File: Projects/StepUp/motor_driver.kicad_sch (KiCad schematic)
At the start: 39 parts, among them J4 AST250404, Q1 BSS84, Q2 2N7002-7-F, U4 TMC2300-LA

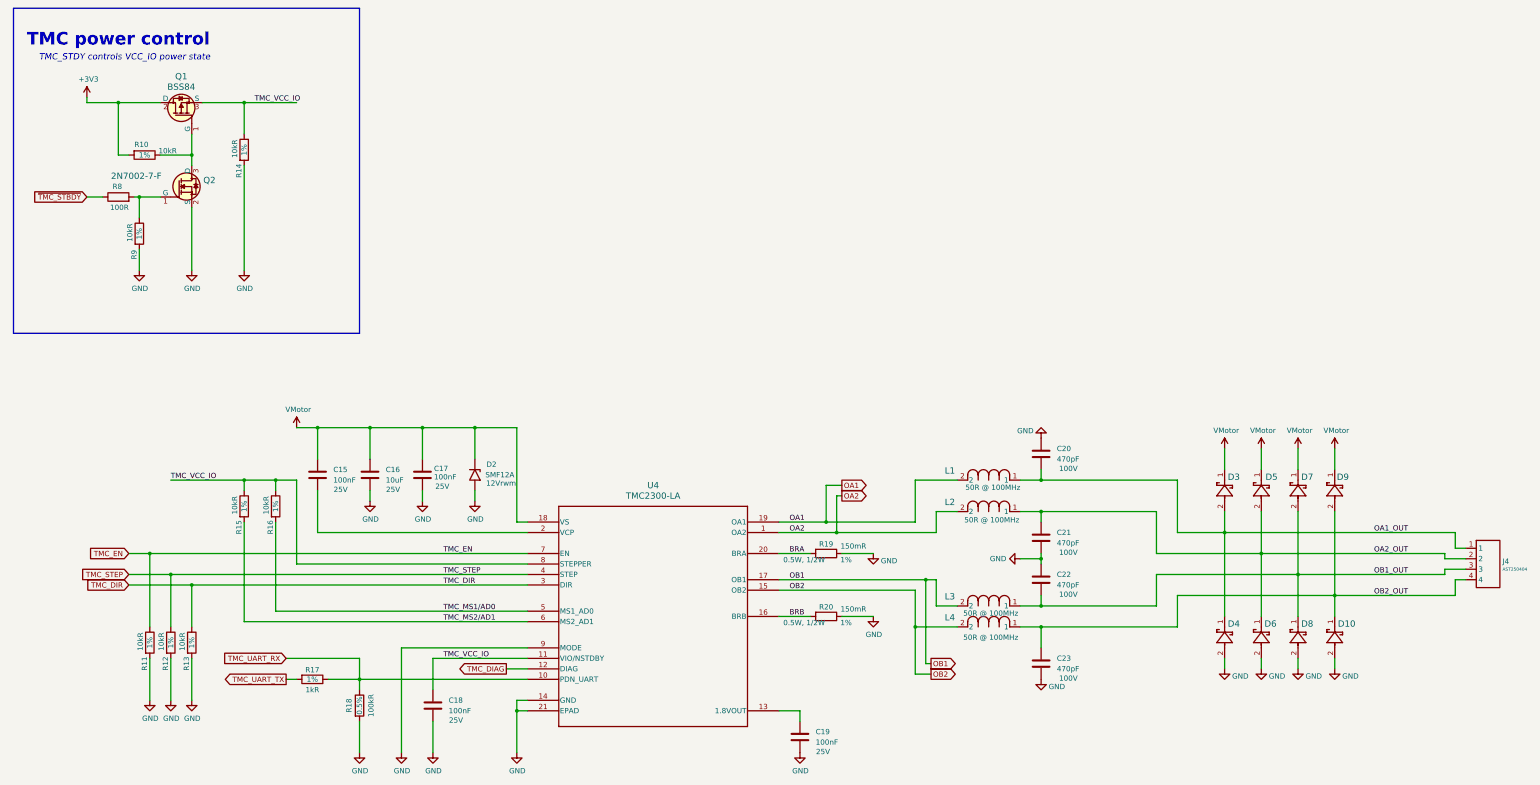
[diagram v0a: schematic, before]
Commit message: feat(layout): Layout begins
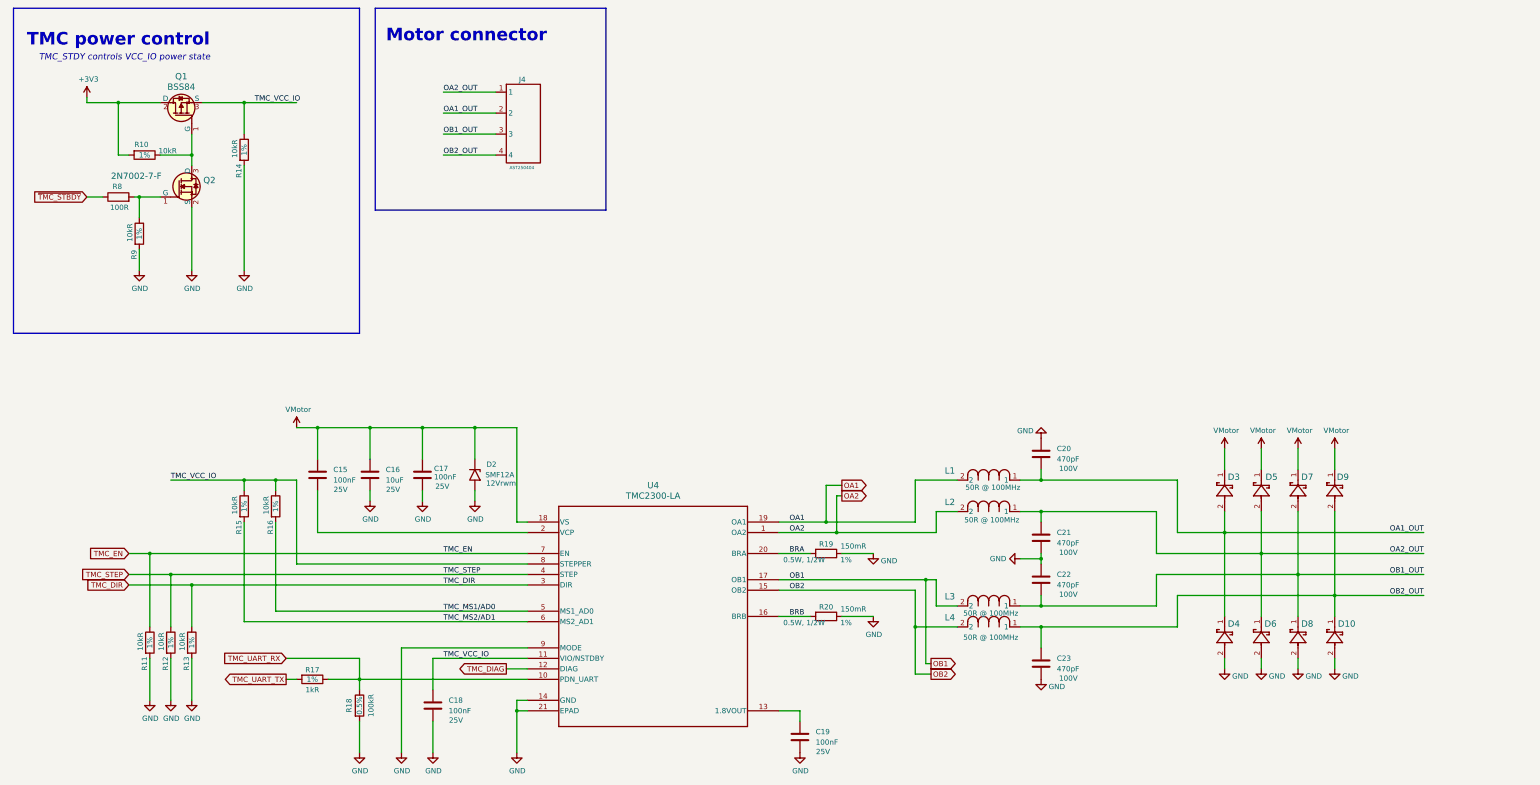
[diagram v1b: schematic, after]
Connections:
- net OA1_OUT: now also J4.2; no longer J4.1
- net OA2_OUT: now also J4.1; no longer J4.2
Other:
- note added: "Motor connector"
